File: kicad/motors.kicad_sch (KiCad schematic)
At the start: 57 parts, among them J12 Conn_01x04_Pin, J3 Conn_01x04_Pin, J4 Conn_01x04_Pin, J5 Conn_01x04_Pin, J6 Conn_01x04_Pin, U3 DRV8825PWP, U4 DRV8825PWP, U5 DRV8825PWP, U6 DRV8825PWP

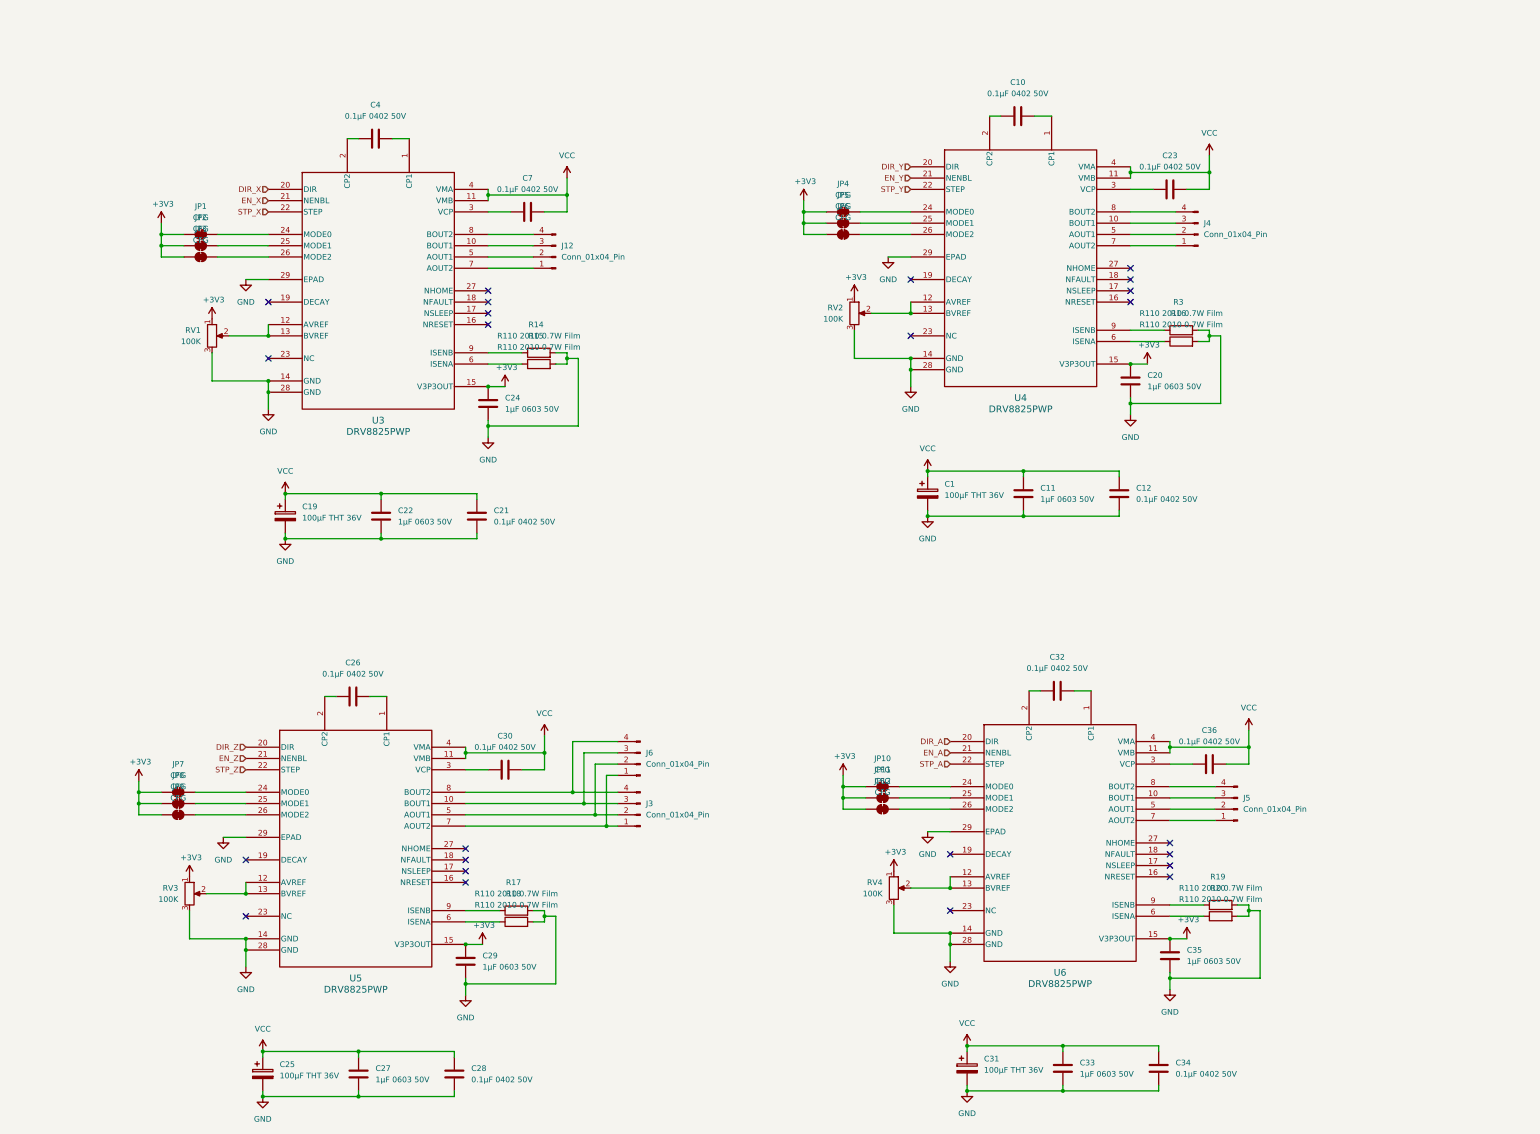
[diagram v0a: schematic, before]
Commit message: PCB redo
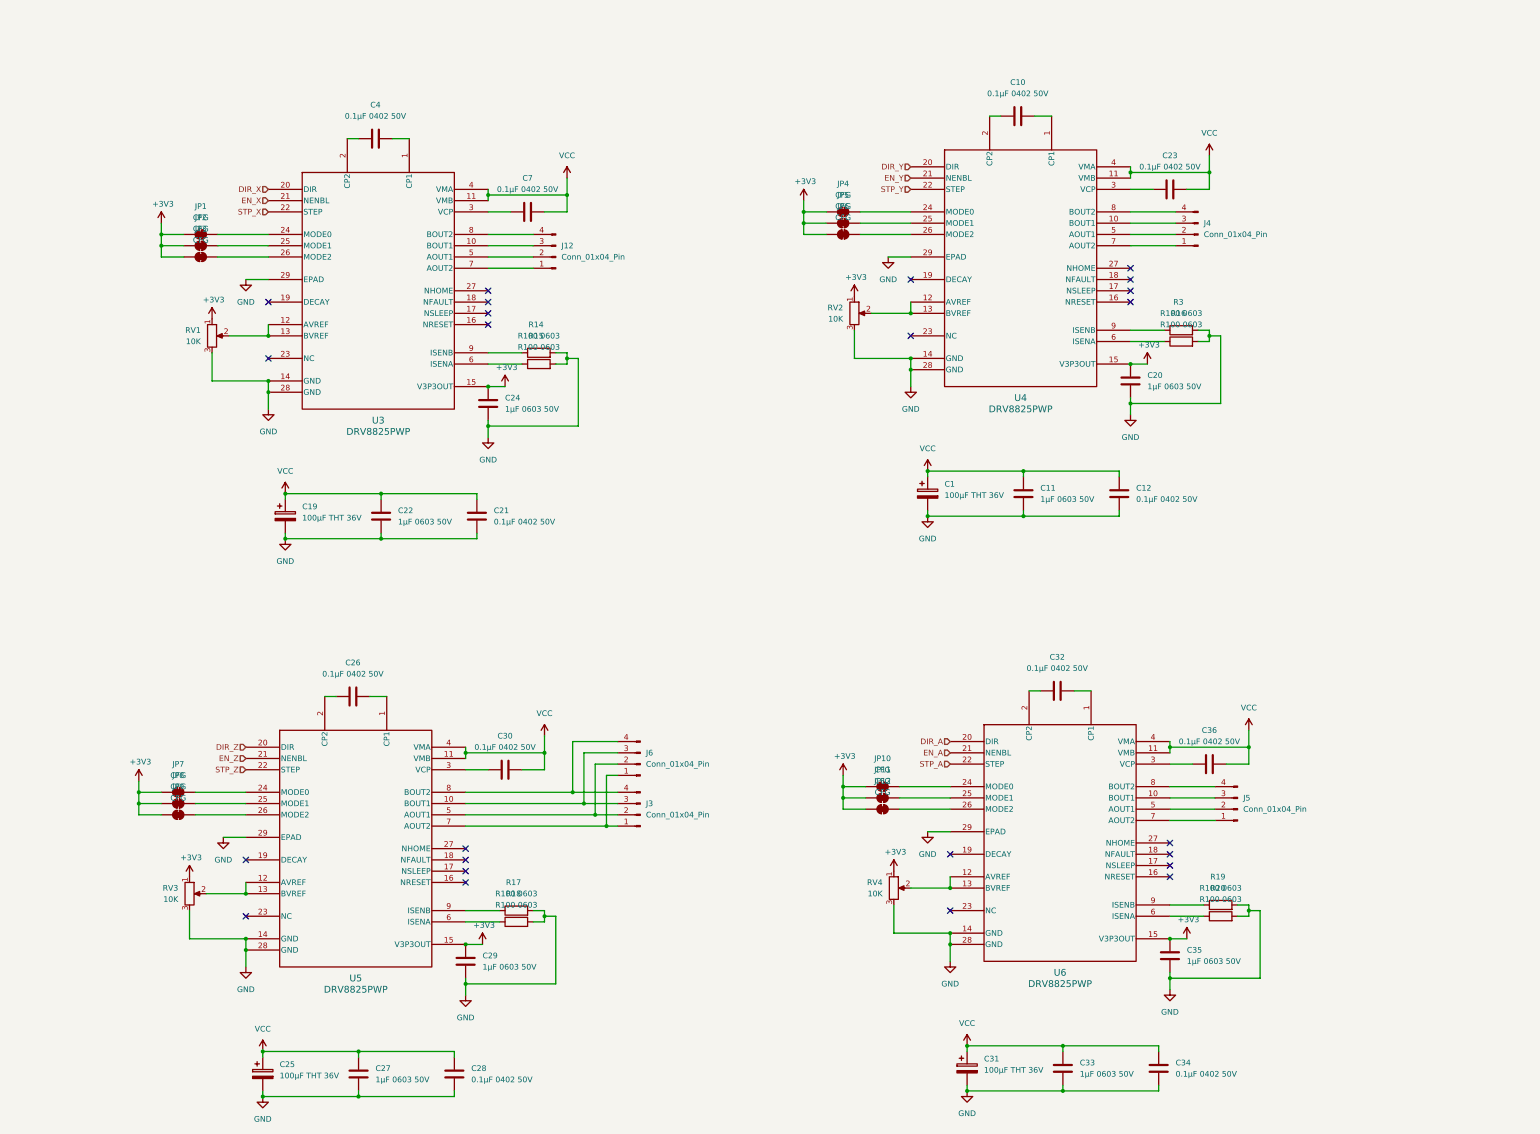
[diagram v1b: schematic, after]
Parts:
- R14, R15, R16, R17, R18, R19, R20, R3: value R110 2010 0.7W Film -> R100 0603; footprint Resistor_SMD:R_2010_5025Metric -> Resistor_SMD:R_0603_1608Metric
- RV1, RV2, RV3, RV4: value 100K -> 10K
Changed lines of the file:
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@@
 			)
 		)
-		(property "Value" "100K"
+		(property "Value" "10K"
 			(at 62.23 93.9799 0)
 			(effects
@@
 			)
 		)
-		(property "Value" "R110 2010 0.7W Film"
+		(property "Value" "R100 0603"
 			(at 138.43 92.71 90)
 			(effects
@@
 			)
 		)
-		(property "Footprint" "Resistor_SMD:R_2010_5025Metric"
+		(property "Footprint" "Resistor_SMD:R_0603_1608Metric"
 			(at 138.43 98.298 90)
 			(effects
@@
 			)
 		)
-		(property "Value" "100K"
+		(property "Value" "10K"
 			(at 57.15 219.7099 0)
 			(effects
@@
 			)
 		)
-		(property "Value" "R110 2010 0.7W Film"
+		(property "Value" "R100 0603"
 			(at 133.35 218.44 90)
 			(effects
@@
 			)
 		)
-		(property "Footprint" "Resistor_SMD:R_2010_5025Metric"
+		(property "Footprint" "Resistor_SMD:R_0603_1608Metric"
 			(at 133.35 224.028 90)
 			(effects
@@
 			)
 		)
-		(property "Value" "100K"
+		(property "Value" "10K"
 			(at 215.9 218.4399 0)
 			(effects
@@
 			)
 		)
-		(property "Value" "R110 2010 0.7W Film"
+		(property "Value" "R100 0603"
 			(at 133.35 220.98 90)
 			(effects
@@
 			)
 		)
-		(property "Footprint" "Resistor_SMD:R_2010_5025Metric"
+		(property "Footprint" "Resistor_SMD:R_0603_1608Metric"
 			(at 133.35 226.568 90)
 			(effects
@@
 			)
 		)
-		(property "Value" "R110 2010 0.7W Film"
+		(property "Value" "R100 0603"
 			(at 138.43 95.25 90)
 			(effects
@@
 			)
 		)
-		(property "Footprint" "Resistor_SMD:R_2010_5025Metric"
+		(property "Footprint" "Resistor_SMD:R_0603_1608Metric"
 			(at 138.43 100.838 90)
 			(effects
@@
 			)
 		)
-		(property "Value" "R110 2010 0.7W Film"
+		(property "Value" "R100 0603"
 			(at 292.1 219.71 90)
 			(effects
@@
 			)
 		)
-		(property "Footprint" "Resistor_SMD:R_2010_5025Metric"
+		(property "Footprint" "Resistor_SMD:R_0603_1608Metric"
 			(at 292.1 225.298 90)
 			(effects
@@
 			)
 		)
-		(property "Value" "R110 2010 0.7W Film"
+		(property "Value" "R100 0603"
 			(at 283.21 90.17 90)
 			(effects
@@
 			)
 		)
-		(property "Footprint" "Resistor_SMD:R_2010_5025Metric"
+		(property "Footprint" "Resistor_SMD:R_0603_1608Metric"
 			(at 283.21 95.758 90)
 			(effects
@@
 			)
 		)
-		(property "Value" "R110 2010 0.7W Film"
+		(property "Value" "R100 0603"
 			(at 292.1 217.17 90)
 			(effects
@@
 			)
 		)
-		(property "Footprint" "Resistor_SMD:R_2010_5025Metric"
+		(property "Footprint" "Resistor_SMD:R_0603_1608Metric"
 			(at 292.1 222.758 90)
 			(effects
@@
 			)
 		)
-		(property "Value" "R110 2010 0.7W Film"
+		(property "Value" "R100 0603"
 			(at 283.21 87.63 90)
 			(effects
@@
 			)
 		)
-		(property "Footprint" "Resistor_SMD:R_2010_5025Metric"
+		(property "Footprint" "Resistor_SMD:R_0603_1608Metric"
 			(at 283.21 93.218 90)
 			(effects
@@
 			)
 		)
-		(property "Value" "100K"
+		(property "Value" "10K"
 			(at 207.01 88.8999 0)
 			(effects

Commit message: schematic candidate 0
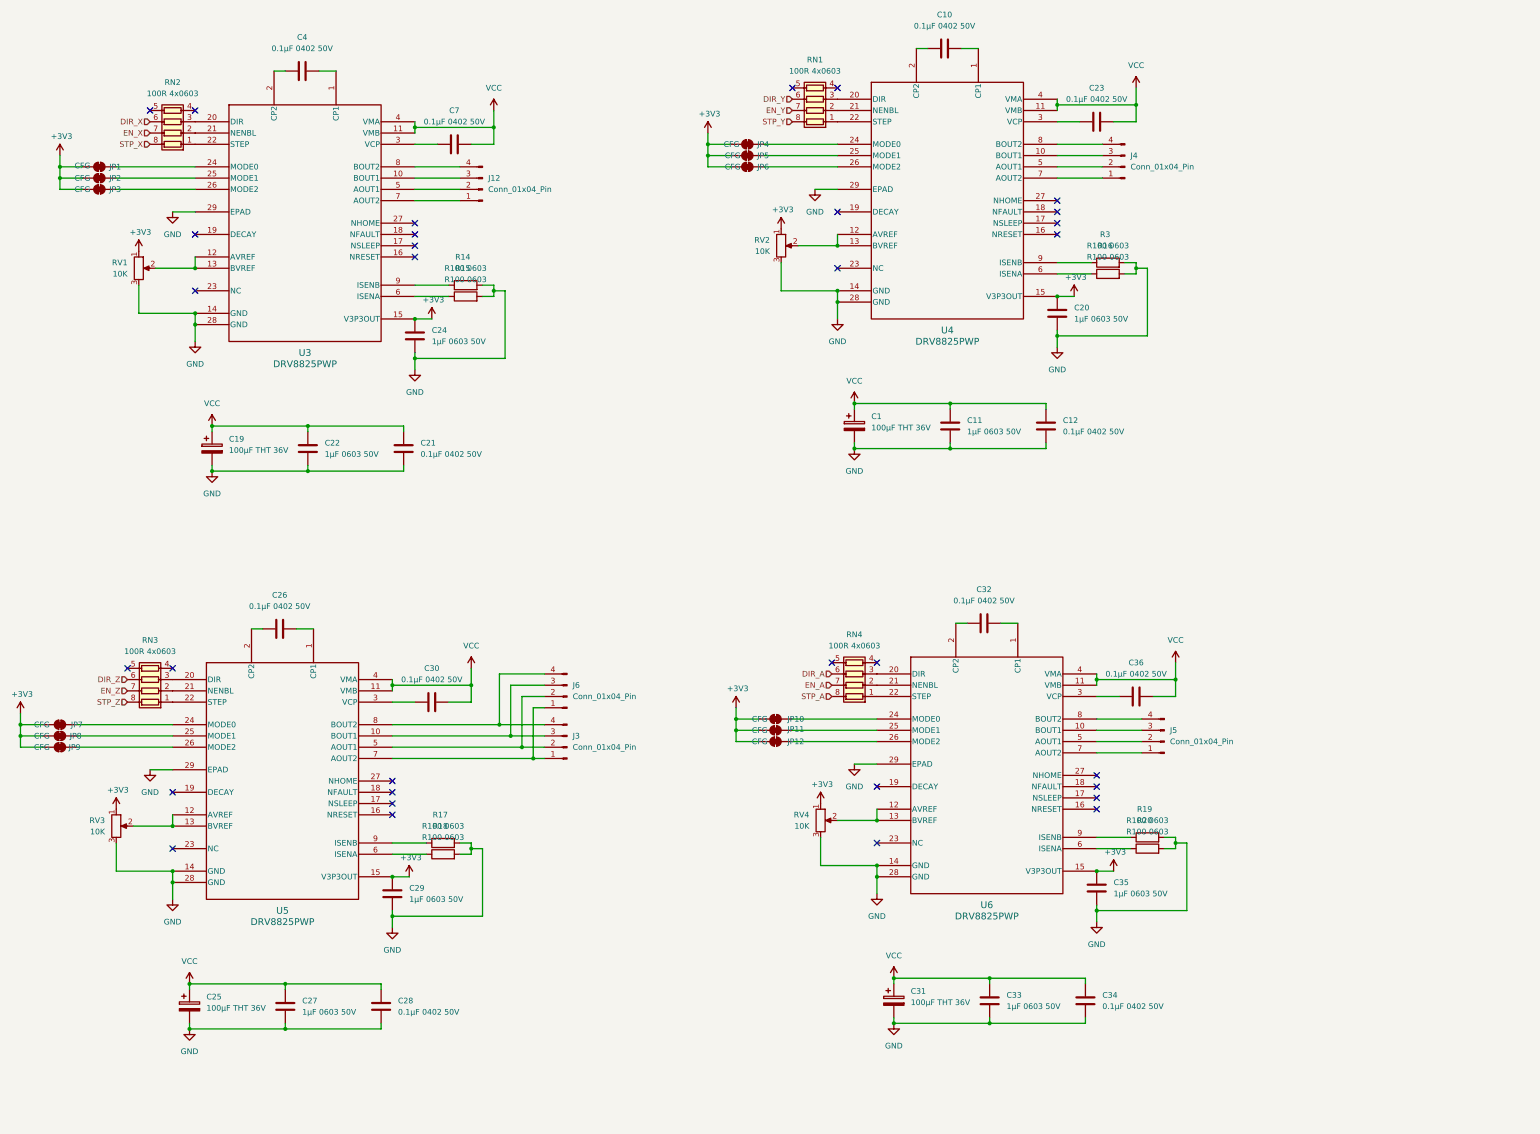
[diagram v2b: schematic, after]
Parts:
- added RN1, RN2, RN3, RN4: 100R 4x0603, Resistor_SMD:R_Array_Concave_4x0603, symbol Device:R_Pack04
- J12, J3, J4, J5, J6: footprint Connector_JST:JST_XH_B4B-XH-A_1x04_P2.50mm_Vertical -> rephat-parts:S4B-XH-SM4-TB
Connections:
- net DIR_A: now also RN4.6 (R3.2); no longer U6.20 (DIR)
- net DIR_X: now also RN2.6 (R3.2); no longer U3.20 (DIR)
- net DIR_Y: now also RN1.6 (R3.2); no longer U4.20 (DIR)
- net DIR_Z: now also RN3.6 (R3.2); no longer U5.20 (DIR)
- net EN_A: now also RN4.7 (R2.2); no longer U6.21 (NENBL)
- net EN_X: now also RN2.7 (R2.2); no longer U3.21 (NENBL)
- net EN_Y: now also RN1.7 (R2.2); no longer U4.21 (NENBL)
- net EN_Z: now also RN3.7 (R2.2); no longer U5.21 (NENBL)
- net STP_A: now also RN4.8 (R1.2); no longer U6.22 (STEP)
- net STP_X: now also RN2.8 (R1.2); no longer U3.22 (STEP)
- net STP_Y: now also RN1.8 (R1.2); no longer U4.22 (STEP)
- net STP_Z: now also RN3.8 (R1.2); no longer U5.22 (STEP)
- new net: RN4.1 (R1.1), U6.22 (STEP)
- new net: RN4.2 (R2.1), U6.21 (NENBL)
- new net: RN4.3 (R3.1), U6.20 (DIR)
- new net: RN3.1 (R1.1), U5.22 (STEP)
- new net: RN3.2 (R2.1), U5.21 (NENBL)
- new net: RN3.3 (R3.1), U5.20 (DIR)
- new net: RN1.1 (R1.1), U4.22 (STEP)
- new net: RN1.2 (R2.1), U4.21 (NENBL)
- new net: RN1.3 (R3.1), U4.20 (DIR)
- new net: RN2.1 (R1.1), U3.22 (STEP)
- new net: RN2.2 (R2.1), U3.21 (NENBL)
- new net: RN2.3 (R3.1), U3.20 (DIR)
- no-connect marks 24 -> 32
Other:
- moved on the sheet: C1, C10, C11, C12, C19, C20, C21, C22, C23, C24, C25, C26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
